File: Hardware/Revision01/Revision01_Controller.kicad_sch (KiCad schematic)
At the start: 4 parts, among them U1 NUCLEO-L476RG, U10 NCP1117LPST50T3G

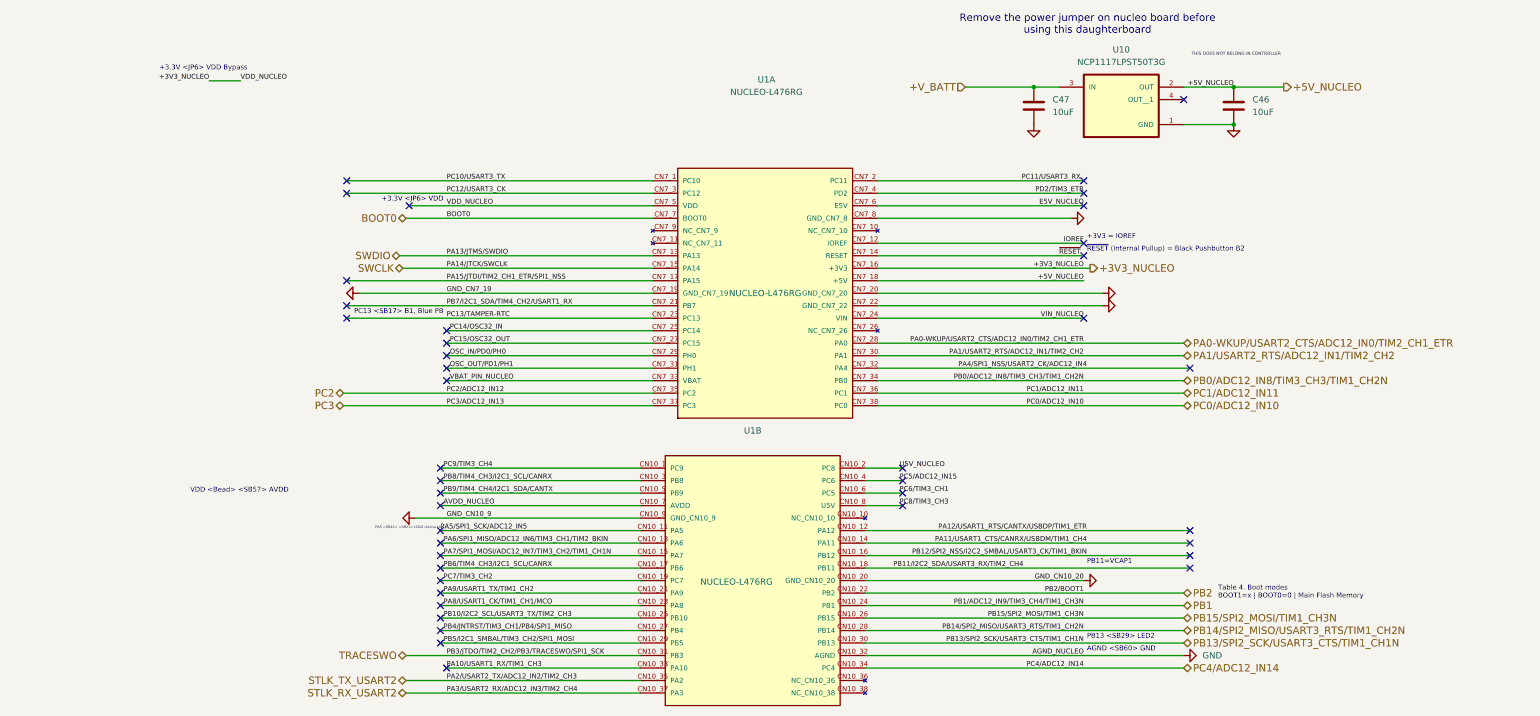
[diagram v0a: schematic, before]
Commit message: implemented feedback
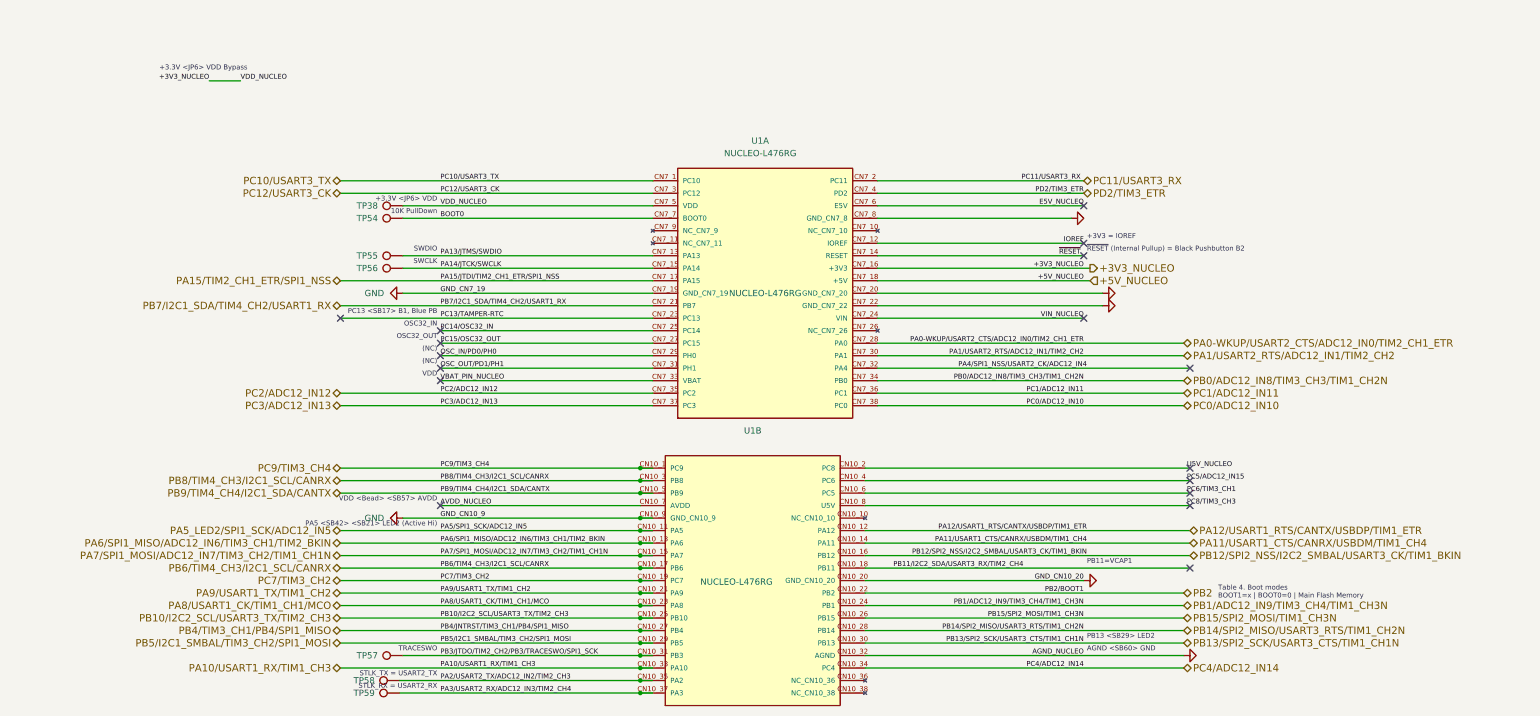
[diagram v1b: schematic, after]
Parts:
- removed C46, C47: 10uF, Capacitor_SMD:C_1206_3216Metric, symbol Device:C
- removed U10: NCP1117LPST50T3G, NCP1117LPST50T3G:SOT230P700X180-4N, symbol NCP1117LPST50T3G:NCP1117LPST50T3G
- added TP38, TP54, TP55, TP56, TP57, TP58, TP59: TestPoint, symbol Connector:TestPoint
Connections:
- net +3V3_NUCLEO: now also TP38.1
- net BOOT0: now also TP54.1
- net PA15/JTDI/TIM2_CH1_ETR/SPI1_NSS renamed PA15/TIM2_CH1_ETR/SPI1_NSS
- net PA5/SPI1_SCK/ADC12_IN5 renamed PA5_LED2/SPI1_SCK/ADC12_IN5
- net PB1 renamed PB1/ADC12_IN9/TIM3_CH4/TIM1_CH3N
- net PB4/JNTRST/TIM3_CH1/PB4/SPI1_MISO renamed PB4/TIM3_CH1/PB4/SPI1_MISO
- net PC2 renamed PC2/ADC12_IN12
- net PC3 renamed PC3/ADC12_IN13
- net STLK_RX_USART2 renamed PA3/USART2_RX/ADC12_IN3/TIM2_CH4
- net PA3/USART2_RX/ADC12_IN3/TIM2_CH4: now also TP59.1
- net STLK_TX_USART2 renamed PA2/USART2_TX/ADC12_IN2/TIM2_CH3
- net PA2/USART2_TX/ADC12_IN2/TIM2_CH3: now also TP58.1
- net SWCLK renamed PA14/JTCK/SWCLK
- net PA14/JTCK/SWCLK: now also TP56.1
- net SWDIO renamed PA13/JTMS/SWDIO
- net PA13/JTMS/SWDIO: now also TP55.1
- net TRACESWO renamed PB3/JTDO/TIM2_CH2/PB3/TRACESWO/SPI1_SCK
- net PB3/JTDO/TIM2_CH2/PB3/TRACESWO/SPI1_SCK: now also TP57.1
- no-connect marks 42 -> 17
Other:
- note added: "(NC)"
- note added: "10K PullDown"
- note added: "OSC32_IN"
- note added: "OSC32_OUT"
- note added: "STLK_RX = USART2_RX"
- note added: "STLK_TX = USART2_TX"
- note added: "SWCLK"
- note added: "SWDIO"
- note added: "TRACESWO"
- note added: "VDD"
- note removed: "Remove the power jumper on nucleo board before using this daughterboard"
- note removed: "THIS DOES NOT BELONG IN CONTROLLER"
